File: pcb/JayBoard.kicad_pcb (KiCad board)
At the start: 2 copper layers, 21 x 51 mm, 33 parts, among them J1 USB_C_Receptacle_USB2.0_14P, J2 Conn_01x20, J3 Conn_01x20, J4 Conn_01x03, SW1 SW_Push, U1 RP2040, U2 W25Q128JVS, U3 MCP1700x-330xxTT, Y1 12 MHz

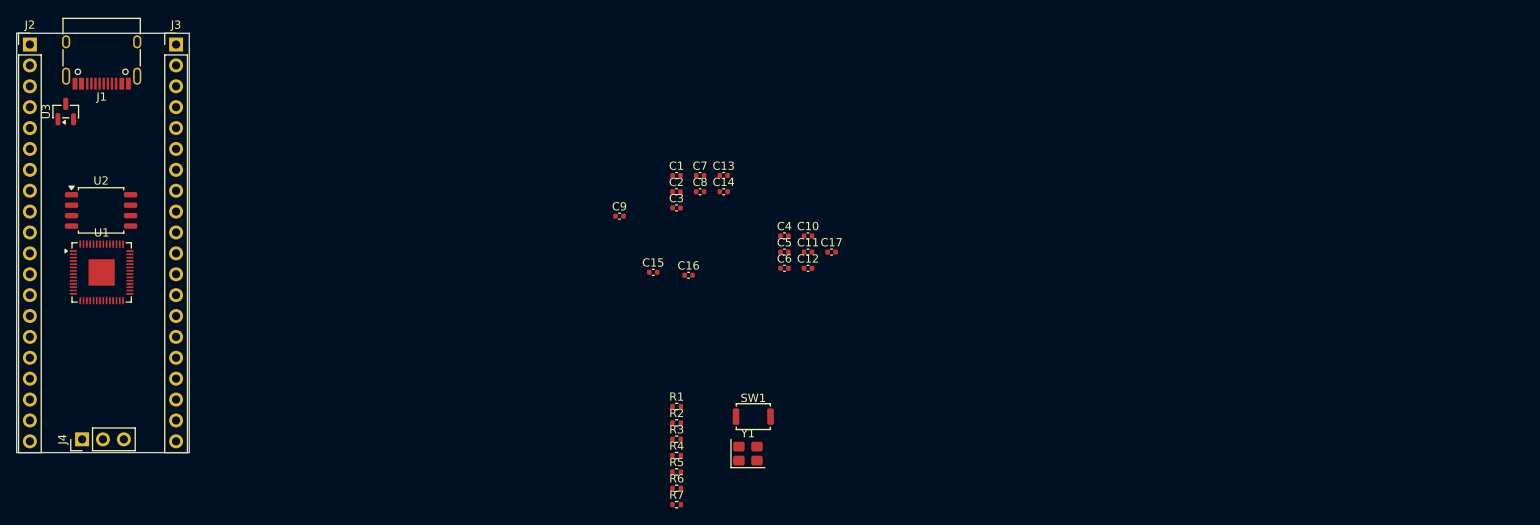
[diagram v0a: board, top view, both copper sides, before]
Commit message: YAY! i did it
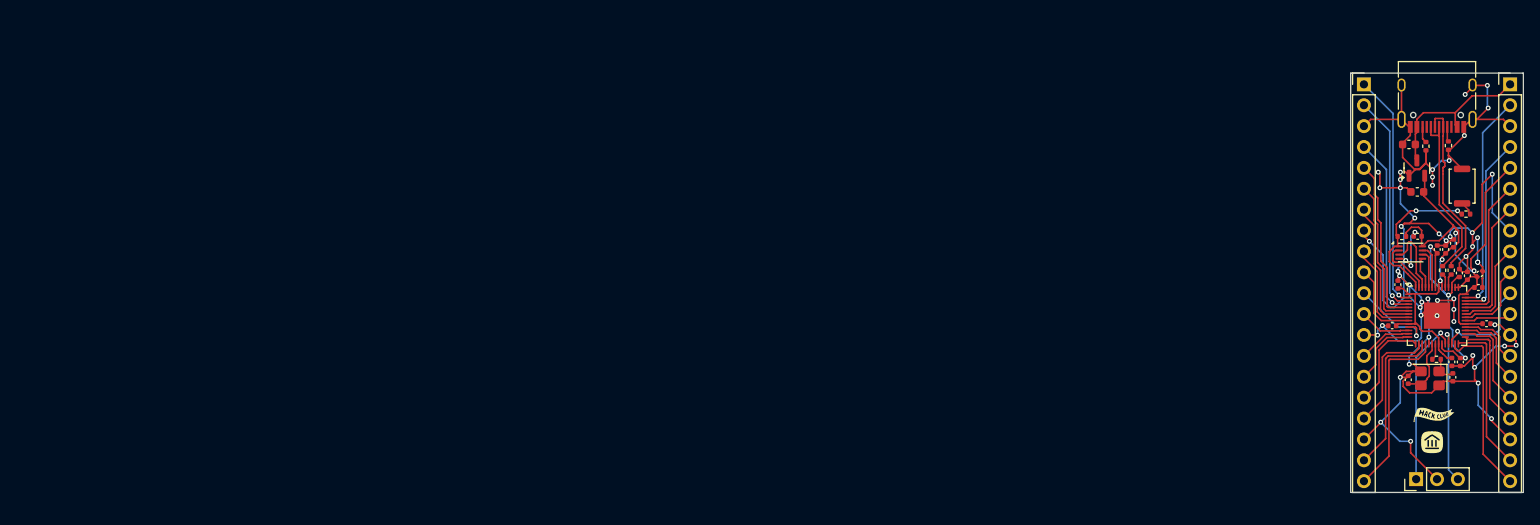
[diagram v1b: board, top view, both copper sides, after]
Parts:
- removed U3: MCP1700x-330xxTT, Package_TO_SOT_SMD:SOT-23
- added G***: LOGO, LOGO, F.Cu at (230.2, 110.8)
- added G***: LOGO, LOGO, F.Cu at (230.5, 107.5)
- added G***: LOGO, LOGO, B.Cu at (230.9, 90.0)
- added U4: W25Q16JVUXIQ TR, Package_SON:Winbond_USON-8-1EP_3x2mm_P0.5mm_EP0.2x1.6mm, F.Cu at (227.6, 87.8)
- C10: value 0.1uF -> 1uF
- C12: value 1uF -> 0.1uF
- C13, C14: footprint Capacitor_SMD:C_0402_1005Metric -> Capacitor_SMD:C_0603_1608Metric
- C15, C16: value 33 pF -> 33pF
- C17: value 0.01 uF -> 0.1uF
- R1: value 5.1k -> 5.1K
- R5: value 1k -> 1K
- R6: value 10k -> 1K
- R7: value 1k -> 10K
- U2: value W25Q128JVS -> MCP1700x-330xxTT; footprint Package_SO:SOIC-8_5.3x5.3mm_P1.27mm -> Package_TO_SOT_SMD:SOT-23
- moved J1 162.5 mm to (230.8, 68.4)
- moved U1 162.5 mm to (230.8, 95.4)
- moved J2 162.3 mm to (221.9, 67.3)
- moved J3 162.3 mm to (239.7, 67.3)
- moved J4 162.3 mm to (228.3, 115.3)
- moved U2 160.1 mm to (228.4, 77.5), turned to 90 degrees
- moved C9 106.3 mm to (236.8, 96.4)
- moved R6 101.6 mm to (234.3, 83.1)
- moved R2 99.7 mm to (232.2, 74.8), turned to -90 degrees
- moved C1 98.4 mm to (236.0, 90.4), turned to 45 degrees
- moved R4 96.9 mm to (232.5, 89.9), turned to -90 degrees
- moved C2 96.5 mm to (232.6, 101.1), turned to -90 degrees
- moved R1 96.5 mm to (229.5, 74.8), turned to -90 degrees
- moved R3 95.4 mm to (231.5, 89.9), turned to -90 degrees
- moved C8 95.4 mm to (235.8, 92.0)
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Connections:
- net USB_D_+ renamed USB_D+
- R1 pad 1: Net-(J1-CC1) -> Net-(J1-CC2)
- R2 pad 1: Net-(J1-CC2) -> Net-(J1-CC1)
- R5 pad 2: unconnected-(R5-Pad2) -> XOUT
- R6 pad 1: +3V3 -> QSPI_SS
- R6 pad 2: QSPI_SS -> Net-(R6-Pad2)
- R7 pad 1: Net-(R7-Pad1) -> QSPI_SS
- R7 pad 2: QSPI_SS -> +3V3
- SW1 pad 2: Net-(R7-Pad1) -> Net-(R6-Pad2)
- U1 pad 19: unconnected-(U1-TESTEN-Pad19) -> GND
- U1 pad 24: unconnected-(U1-SWCLK-Pad24) -> SWCLK
- U1 pad 25: unconnected-(U1-SWD-Pad25) -> SWD
- U1 pad 26: unconnected-(U1-RUN-Pad26) -> RUN
- U2 pad 1: QSPI_SS -> GND
- U2 pad 2: QSPI_SD1 -> +3V3
- U2 pad 3: QSPI_SD2 -> VBUS
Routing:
- net GND: track 0.00 -> 257.1 mm, vias 0 -> 55
- net +3V3: track 0.00 -> 81.2 mm, vias 0 -> 4
- net +1V1: track 0.00 -> 30.9 mm, vias 0 -> 3
- net GPIO0: track 0.00 -> 28.7 mm, vias 0 -> 1
- net GPIO1: track 0.00 -> 26.9 mm, vias 0 -> 1
- net GPIO29_ADC3: track 0.00 -> 26.4 mm, vias 0 -> 1
- net GPIO2: track 0.00 -> 22.4 mm, vias 0 -> 1
- net GPIO28_ADC2: track 0.00 -> 22.2 mm, vias 0 -> 1
- net USB_D+: track 0.00 -> 22.1 mm
- net USB_D-: track 0.00 -> 22.0 mm
- net GPIO16: track 0.00 -> 22.0 mm
- net GPIO15: track 0.00 -> 21.8 mm
- net GPIO3: track 0.00 -> 20.7 mm
- net SWCLK: track 0.00 -> 20.6 mm, vias 0 -> 1
- net VBUS: track 0.00 -> 20.1 mm
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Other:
- board text added: "Jaytirt Joshi"
- board text added: "Joshi1.com/JayBoard"
